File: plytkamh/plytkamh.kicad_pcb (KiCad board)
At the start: 2 copper layers, 70 x 50 mm, 57 parts, among them J1 USB_C_Receptacle_USB2.0_16P, J2 BOOT0, J3 Conn_01x06, J4 COMM, J5 ANALOG_GPIO, Q1 TEMT6000X01, SW1 RESET, SW2 USER, U1 USBLC6-2SC6, U2 LDL1117S33R, U3 STM32F446RETx, U4 BME280, Y1 12MHz

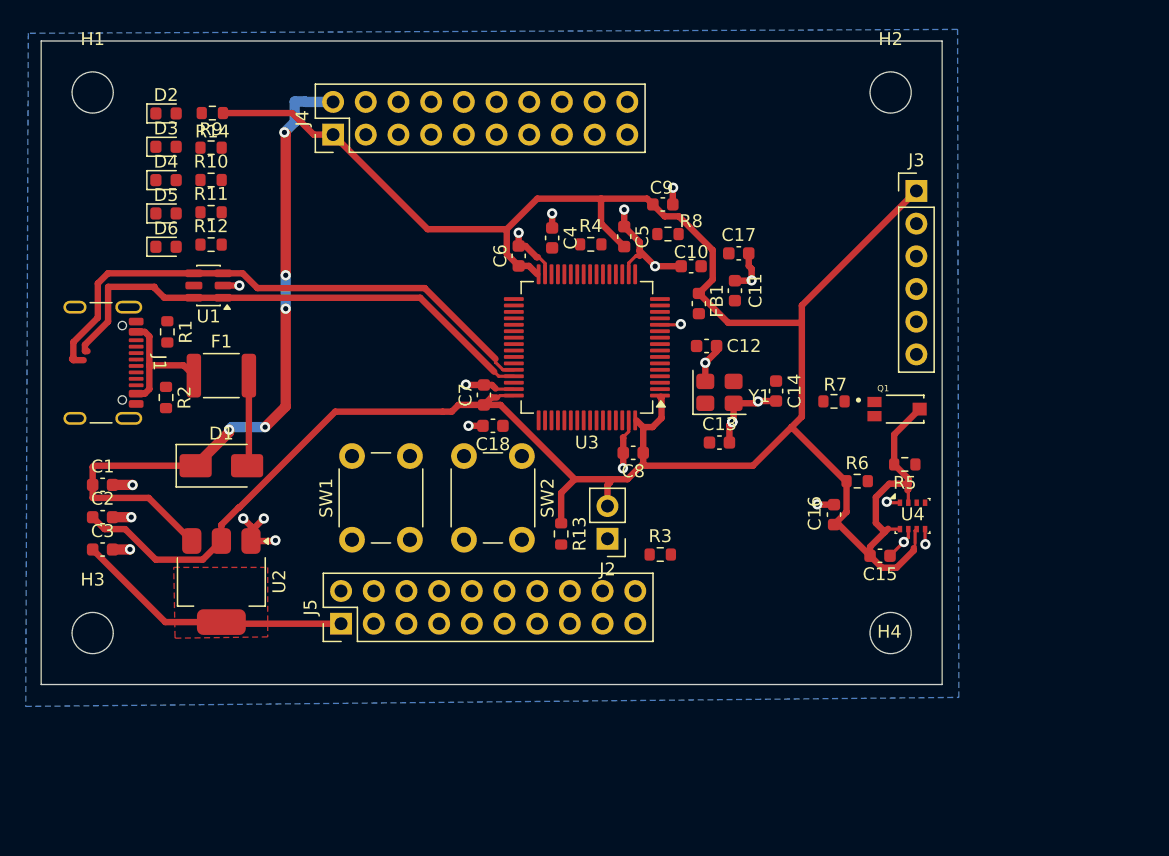
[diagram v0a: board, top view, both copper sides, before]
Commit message: after resizing
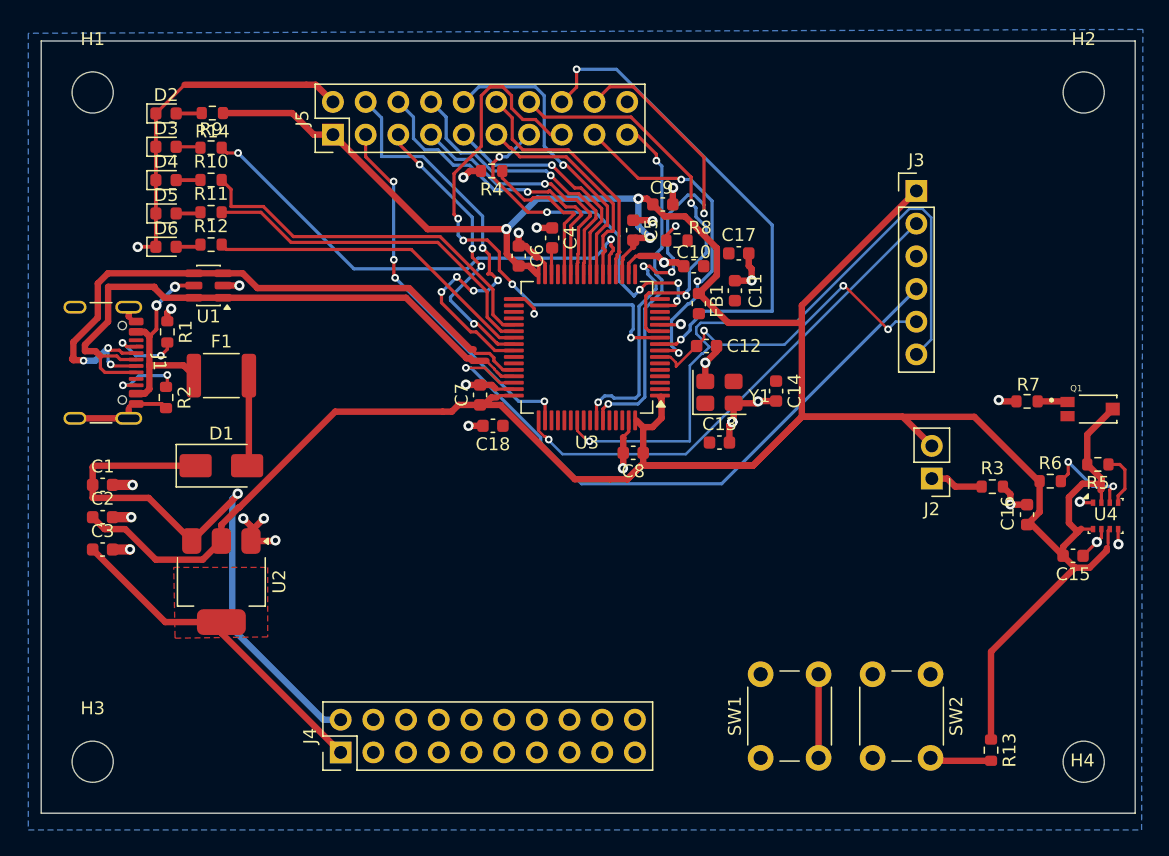
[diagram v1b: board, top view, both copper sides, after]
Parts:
- moved J4 48.0 mm to (123.3, 155.3)
- moved J5 38.0 mm to (122.7, 107.3)
- moved R13 37.4 mm to (173.8, 155.1)
- moved SW1 36.0 mm to (155.9, 155.7)
- moved SW2 36.0 mm to (169.1, 149.2)
- moved R3 26.3 mm to (173.9, 134.6)
- moved J2 25.6 mm to (169.2, 134.0)
- moved H4 18.0 mm to (181.0, 156.0)
- moved C15 15.0 mm to (180.2, 140.0)
- moved C16 15.0 mm to (176.6, 136.8)
- moved H2 15.0 mm to (181.0, 104.0)
- moved Q1 15.0 mm to (181.5, 128.6)
- moved R5 15.0 mm to (182.1, 132.9)
- moved R6 15.0 mm to (178.4, 134.2)
- moved R7 15.0 mm to (176.6, 128.0)
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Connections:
- J5 pad 10: PA4 -> PA7
- J5 pad 11: PB0 -> PA6
- J5 pad 12: PB1 -> PA4
- J5 pad 13: PA6 -> PA1
- J5 pad 14: PA7 -> PC3
- J5 pad 15: PA8 -> PC2
- J5 pad 16: PA15 -> PC1
- J5 pad 17: PB6 -> PC0
- J5 pad 18: PB7 -> PB6
- J5 pad 19: PC9 -> PB7
- J5 pad 3: PC0 -> PA15
- J5 pad 4: PC1 -> PA8
- J5 pad 5: PC2 -> PC9
- J5 pad 6: PC3 -> PB1
- J5 pad 7: PC4 -> PB0
- J5 pad 9: PA1 -> PC4
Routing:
- net +3.3V: track 229.8 -> 289.7 mm, vias 0 -> 3
- net SWO: track 0.00 -> 53.3 mm, vias 0 -> 1
- net SWDIO: track 0.00 -> 49.4 mm, vias 0 -> 1
- net PB6: track 0.00 -> 43.1 mm, vias 0 -> 4
- net PC2: track 0.00 -> 42.1 mm, vias 0 -> 4
- net PC1: track 0.00 -> 39.9 mm, vias 0 -> 2
- net GND: track 58.4 -> 97.8 mm, vias 25 -> 29
- net SWCLK: track 0.00 -> 38.4 mm, vias 0 -> 1
- net LED_STATUS: track 0.00 -> 38.1 mm, vias 0 -> 2
- net PA8: track 0.00 -> 34.0 mm, vias 0 -> 5
- net NRST: track 0.00 -> 32.4 mm, vias 0 -> 3
- net PC3: track 0.00 -> 32.4 mm, vias 0 -> 2
- net LED_USER_1: track 0.00 -> 29.3 mm
- net PA15: track 0.00 -> 29.3 mm, vias 0 -> 4
- net PA1: track 0.00 -> 28.6 mm, vias 0 -> 5
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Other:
- board size 70 x 50 mm -> 85 x 60 mm
